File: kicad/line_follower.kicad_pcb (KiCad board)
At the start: 2 copper layers, 80 x 100 mm, 39 parts, among them J1 XT30PW-M, M1 MOTOR_ENC, M2 MOTOR_ENC, Q1 ALS-PT19-315C_L177_TR8, Q2 ALS-PT19-315C_L177_TR8, Q3 ALS-PT19-315C_L177_TR8, Q4 ALS-PT19-315C_L177_TR8, Q5 ALS-PT19-315C_L177_TR8, SW1 SW_Push, U1 A4950E, U2 A4950E, U3 NCV4274CDT50RKG, X1 ESP32_DEVKITV1, X2 GY-521-module, X3 DISTANCE_SENSOR

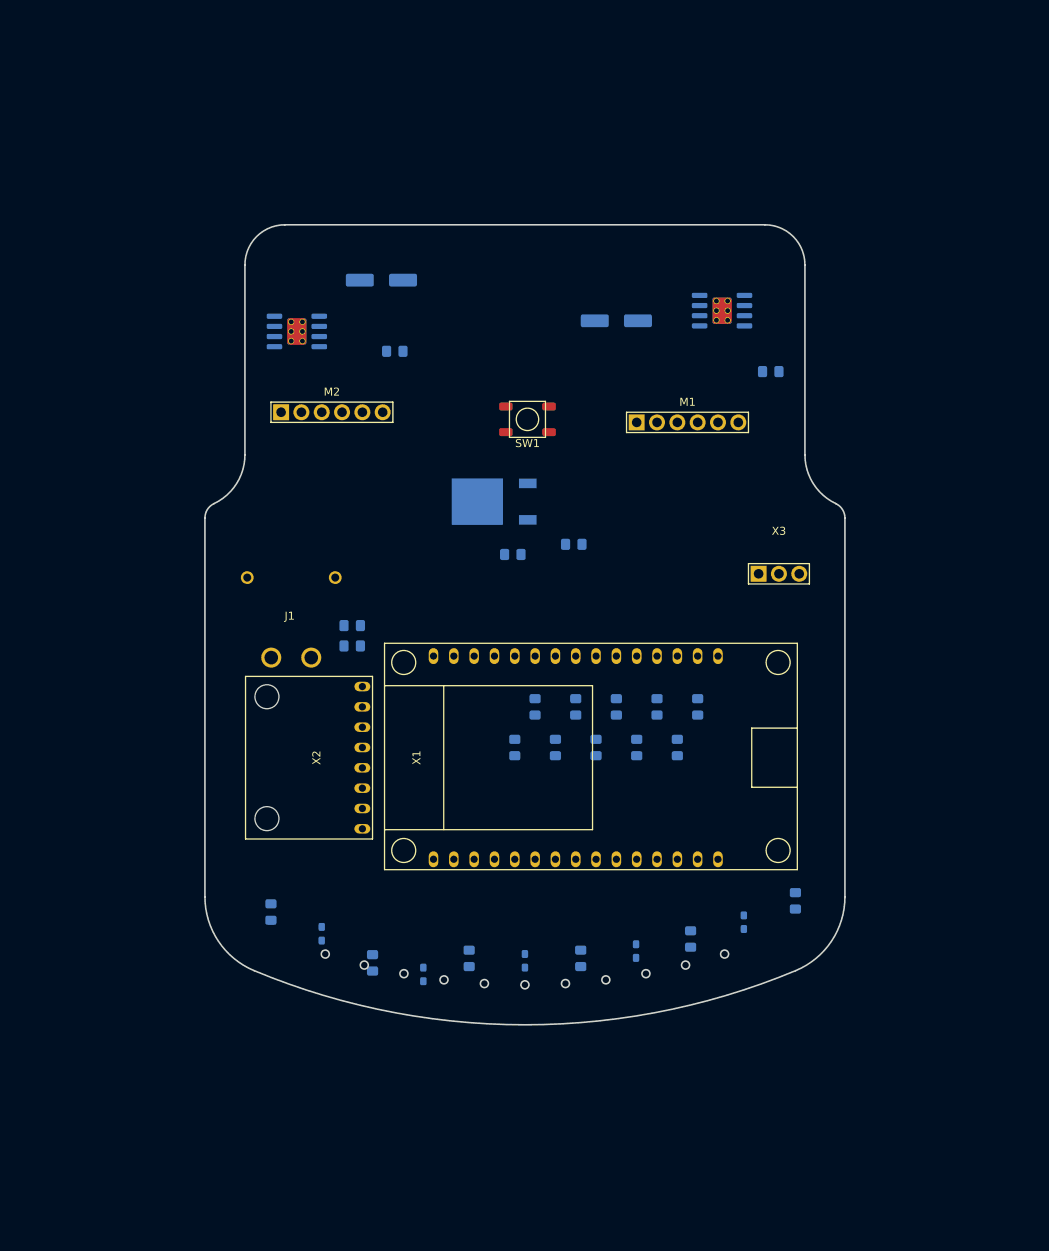
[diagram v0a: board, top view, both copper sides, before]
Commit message: Getting there with the PCB design.
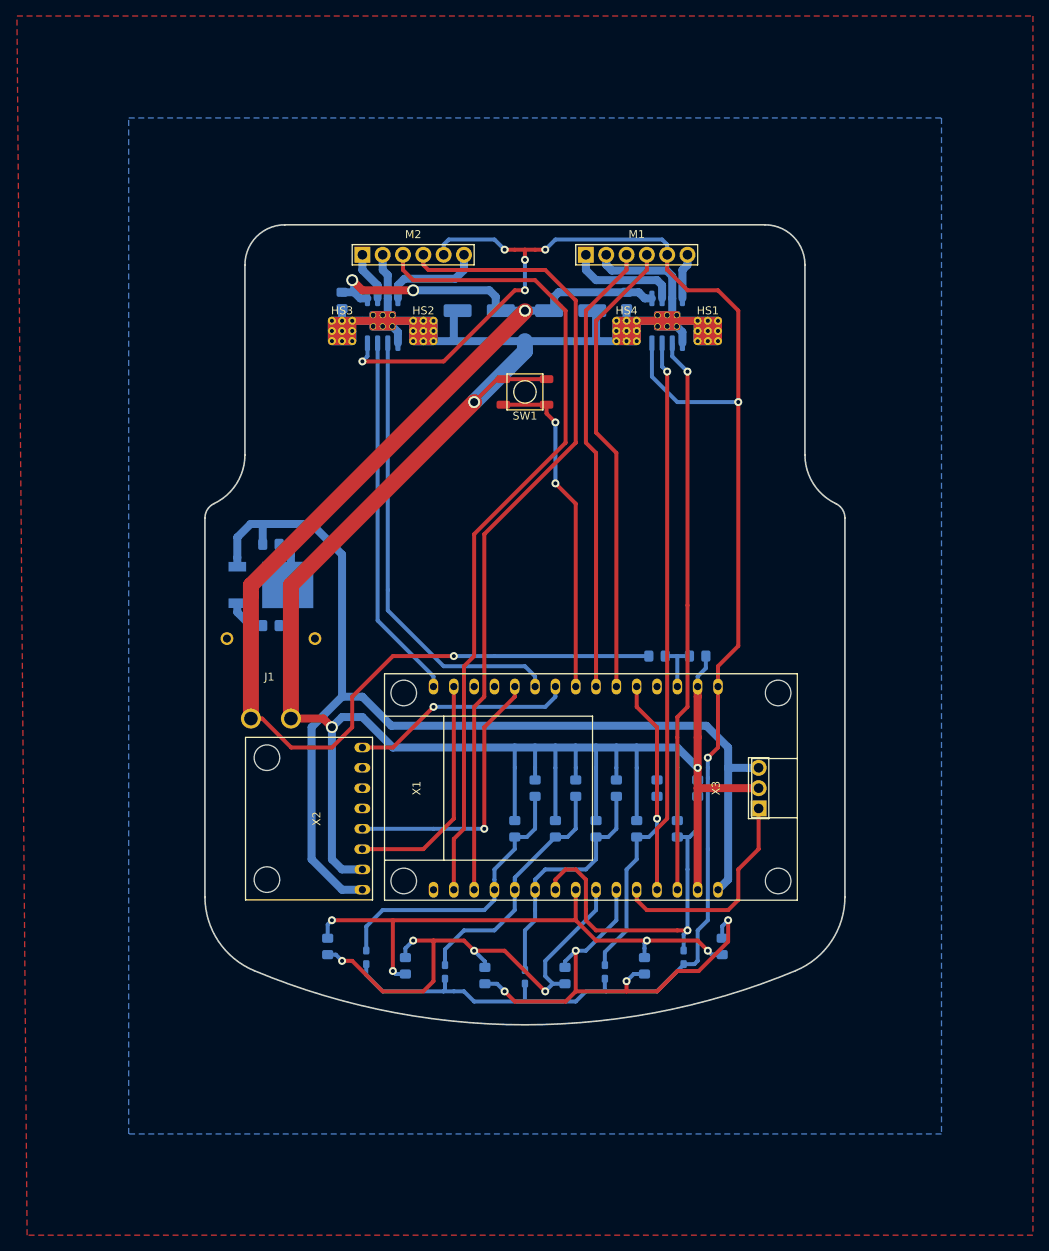
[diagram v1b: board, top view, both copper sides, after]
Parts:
- added HS1: Heatsink_Pad, cube-library:3x3_thermal_vias, F.Cu at (22.9, 1.27)
- added HS2: Heatsink_Pad, cube-library:3x3_thermal_vias, F.Cu at (-12.7, 1.27)
- added HS3: Heatsink_Pad, cube-library:3x3_thermal_vias, F.Cu at (-22.9, 1.27)
- added HS4: Heatsink_Pad, cube-library:3x3_thermal_vias, F.Cu at (12.7, 1.27)
- moved R7 43.2 mm to (21.6, 41.9), turned to 0 degrees
- moved C10 39.2 mm to (-31.8, 38.1)
- moved R6 38.3 mm to (16.5, 41.9)
- moved C11 30.3 mm to (-31.8, 27.9)
- moved U3 29.8 mm to (-31.8, 33.0), turned to 0 degrees
- moved X3 26.9 mm to (29.2, 58.4), turned to 90 degrees
- moved M2 22.2 mm to (-14.0, -8.26)
- moved M1 21.9 mm to (14.0, -8.26)
- moved C6 20.1 mm to (12.7, -2.54), turned to 270 degrees
- moved C9 12.8 mm to (-5.71, -1.27), turned to 180 degrees
- moved U2 10.8 mm to (-17.8, 0.00), turned to 90 degrees
- moved D1 10.8 mm to (24.7, 78.2)
- moved R1 10.2 mm to (21.6, 58.4)
- moved R2 10.2 mm to (16.5, 58.4)
- moved R3 10.2 mm to (11.4, 58.4)
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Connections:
- net /LINE_SENSOR1 renamed LINE_SENSOR1
- net /LINE_SENSOR2 renamed LINE_SENSOR2
- C1 pad 2: /LINE_SENSOR0 -> LINE_SENSOR0
- C4 pad 2: /LINE_SENSOR3 -> LINE_SENSOR3
- C5 pad 2: /LINE_SENSOR4 -> LINE_SENSOR4
- D1 pad 1: /LINE_LED1 -> LINE_LED1
- D1 pad 2: /LINE_LED0 -> LINE_LED0
- D2 pad 1: /LINE_LED0 -> LINE_LED0
- D2 pad 2: /LINE_LED1 -> LINE_LED1
- D3 pad 1: /LINE_LED2 -> LINE_LED2
- D3 pad 2: /LINE_LED0 -> LINE_LED0
- D4 pad 1: /LINE_LED0 -> LINE_LED0
- D4 pad 2: /LINE_LED2 -> LINE_LED2
- D5 pad 1: /LINE_LED1 -> LINE_LED1
- D5 pad 2: /LINE_LED2 -> LINE_LED2
- D6 pad 1: /LINE_LED2 -> LINE_LED2
- D6 pad 2: /LINE_LED1 -> LINE_LED1
- Q1 pad 2: /LINE_SENSOR0 -> LINE_SENSOR0
- Q4 pad 2: /LINE_SENSOR3 -> LINE_SENSOR3
- Q5 pad 2: /LINE_SENSOR4 -> LINE_SENSOR4
- R1 pad 2: /LINE_SENSOR0 -> LINE_SENSOR0
- R4 pad 2: /LINE_SENSOR3 -> LINE_SENSOR3
- R5 pad 2: /LINE_SENSOR4 -> LINE_SENSOR4
- U1 pad 4: +5V -> +3V3
- U2 pad 4: +5V -> +3V3
- X1 pad 10: /LINE_LED2 -> LINE_LED0
- X1 pad 11: /LINE_SENSOR3 -> /RANGE
- X1 pad 12: /MOTOR2A -> /MOTOR1B
- X1 pad 13: /MOTOR2B -> /MOTOR1A
- X1 pad 2: /ENCODER1B -> /ENCODER2A
- X1 pad 21: /ENCODER2B -> /ENCODER1A
- X1 pad 22: /ENCODER2A -> /ENCODER1B
- X1 pad 25: /MOTOR1A -> /MOTOR2B
- X1 pad 3: /ENCODER1A -> /ENCODER2B
- X1 pad 30: /MOTOR1B -> /MOTOR2A
- X1 pad 4: /LINE_SENSOR0 -> LINE_SENSOR4
- X1 pad 5: /RANGE -> LINE_SENSOR3
- X1 pad 7: /LINE_SENSOR4 -> LINE_SENSOR0
- X1 pad 8: /LINE_LED0 -> LINE_LED1
- X1 pad 9: /LINE_LED1 -> LINE_LED2
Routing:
- net GND: track 0.00 -> 415.5 mm, vias 0 -> 3
- net +3V3: track 0.00 -> 228.1 mm, vias 0 -> 7
- net +BATT: track 0.00 -> 187.5 mm, vias 0 -> 4
- net +5V: track 0.00 -> 142.3 mm
- net /ENCODER2A: track 0.00 -> 102.5 mm
- net /ENCODER2B: track 0.00 -> 101.1 mm
- net /MOTOR1A: track 0.00 -> 69.6 mm, vias 0 -> 1
- net /MOTOR1B: track 0.00 -> 69.1 mm, vias 0 -> 1
- net LINE_LED1: track 0.00 -> 68.2 mm, vias 0 -> 4
- net LINE_LED2: track 0.00 -> 62.7 mm, vias 0 -> 4
- net LINE_LED0: track 0.00 -> 61.7 mm, vias 0 -> 4
- net /ENCODER1A: track 0.00 -> 57.7 mm
- net /ENCODER1B: track 0.00 -> 56.6 mm
- net /MOTOR2B: track 0.00 -> 56.5 mm
- net /MOTOR2A: track 0.00 -> 45.8 mm
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- added copper zone on B.Cu, net GND
- added copper zone on F.Cu, net GND
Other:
- outline, holes or cut-outs redrawn

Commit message: Board done except for the motor mounts
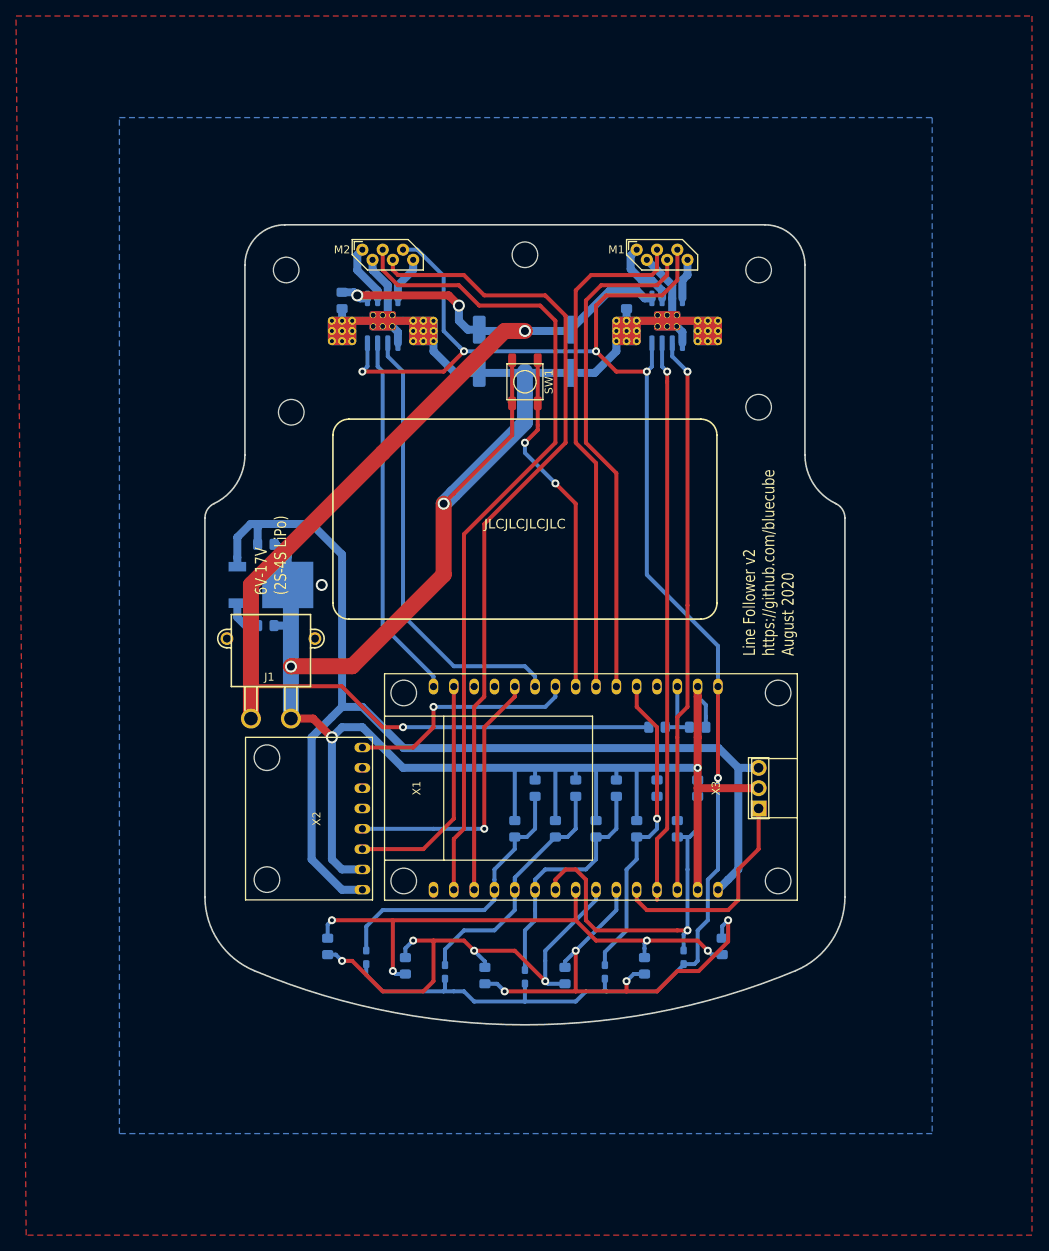
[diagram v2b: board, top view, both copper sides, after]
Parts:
- added H1: MountingHole, MountingHole:MountingHole_3.2mm_M3, F.Cu at (0.00, -8.26)
- added H2: MountingHole, MountingHole:MountingHole_3.2mm_M3, F.Cu at (-29.8, -6.35)
- added H3: MountingHole, MountingHole:MountingHole_3.2mm_M3, F.Cu at (-29.2, 11.4)
- added H4: MountingHole, MountingHole:MountingHole_3.2mm_M3, F.Cu at (29.2, -6.35)
- added H5: MountingHole, MountingHole:MountingHole_3.2mm_M3, F.Cu at (29.2, 10.8)
- M1, M2: footprint cube-library:SolderWirePad1x6_p2.54 -> cube-library:SolderWirePad2x3_p2.54_staggered
- moved R6 8.89 mm to (16.5, 50.8)
- moved R7 8.89 mm to (21.6, 50.8)
- moved C8 5.08 mm to (5.71, 3.81), turned to 270 degrees
- moved C9 5.08 mm to (-5.71, 3.81), turned to 270 degrees
- moved M2 3.86 mm to (-17.8, -8.89)
- moved M1 2.62 mm to (16.5, -8.89)
- moved SW1 1.27 mm to (0.00, 7.62), turned to 270 degrees
- moved C10 0.63 mm to (-32.4, 38.1)
- moved C11 0.63 mm to (-32.4, 27.9)
- renumbered HS4 to HS2, HS2 to HS4
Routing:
- net GND: track 415.5 -> 381.6 mm, vias 3 -> 5
- net +3V3: track 228.1 -> 213.4 mm, vias 7 -> 5
- net +BATT: track 187.5 -> 178.9 mm
- net /ENCODER1B: track 56.6 -> 64.3 mm
- net Net-(M2-Pad6): track 12.0 -> 5.61 mm
- net /ENCODER1A: track 57.7 -> 63.2 mm
- net Net-(M1-Pad1): track 13.9 -> 8.76 mm
- net /BUTTON: track 42.1 -> 44.1 mm
- net Net-(M2-Pad1): track 5.61 -> 7.41 mm
- net LINE_LED0: track 61.7 -> 59.9 mm
- net LINE_LED2: track 62.7 -> 61.2 mm
- net /ACCEL_INT: track 28.0 -> 29.5 mm
- net +5V: track 142.3 -> 140.9 mm
- net /MOTOR1B: track 69.1 -> 70.4 mm
- net /BAT_SENSE: track 6.84 -> 8.11 mm
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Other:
- board text added: "6V-17V (2S-4S LiPo)"
- board text added: "JLCJLCJLCJLC"
- board text added: "Line Follower v2 https://github.com/bluecube August 2020"
